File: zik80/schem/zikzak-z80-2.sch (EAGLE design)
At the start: 66 parts, among them IC1 Z80, IC10 74LS32N, IC11 74LS32N, IC12 74LS32N, IC13 74LS32N, IC14 74LS04N, IC15 74LS32N, IC16 ATMEGA644-20PU, IC2 ATMEGA644-20PU, IC3 MC6850, IC4 74LS32N, IC5 74LS04N, IC6 74LS32N, U2 FT232RLSSOP, X2 USB-SMD-NS

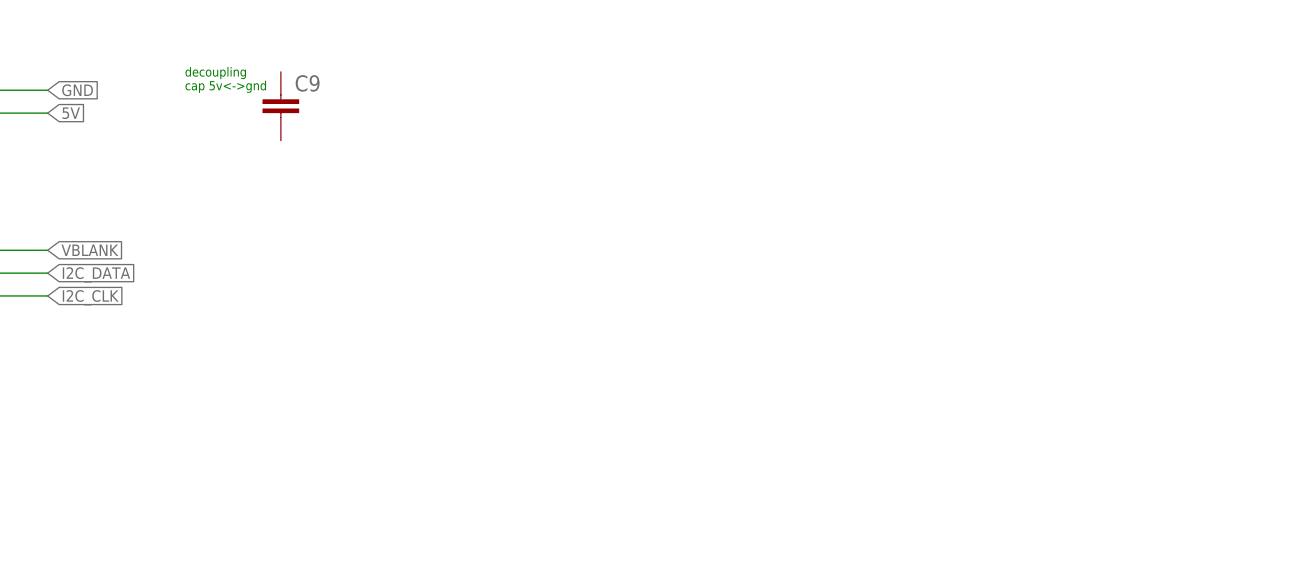
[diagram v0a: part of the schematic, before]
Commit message: Schematic update
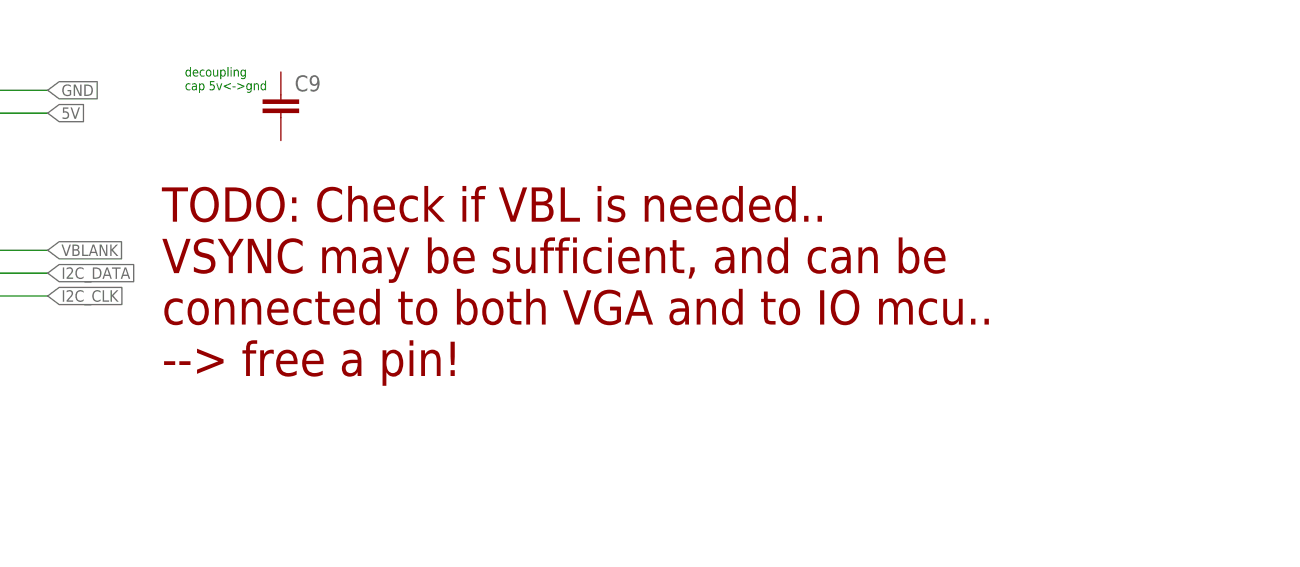
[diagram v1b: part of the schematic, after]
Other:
- note added: "TODO: Check if VBL is needed.. VSYNC may be sufficient, and can be connected to both VGA and to IO mcu.. --> free a pin!"
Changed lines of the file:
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@@
 <setting verticaltext="up"/>
 </settings>
-<grid distance="0.05" unitdist="inch" unit="inch" style="dots" multiple="1" display="yes" altdistance="0.01" altunitdist="inch" altunit="inch"/>
+<grid distance="0.1" unitdist="inch" unit="inch" style="lines" multiple="1" display="no" altdistance="0.01" altunitdist="inch" altunit="inch"/>
 <layers>
 <layer number="1" name="Top" color="4" fill="1" visible="no" active="no"/>
@@
 <rectangle x1="3.81" y1="109.22" x2="35.56" y2="135.89" layer="203"/>
 <text x="6.35" y="138.43" size="5.08" layer="91">ISP Progr. IO</text>
+<text x="478.79" y="40.64" size="3.81" layer="94">TODO: Check if VBL is needed..
+VSYNC may be sufficient, and can be
+connected to both VGA and to IO mcu..
+--&gt; free a pin!</text>
 </plain>
 <instances>
